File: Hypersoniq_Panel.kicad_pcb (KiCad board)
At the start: 2 copper layers, 40.4 x 128.5 mm, 17 parts

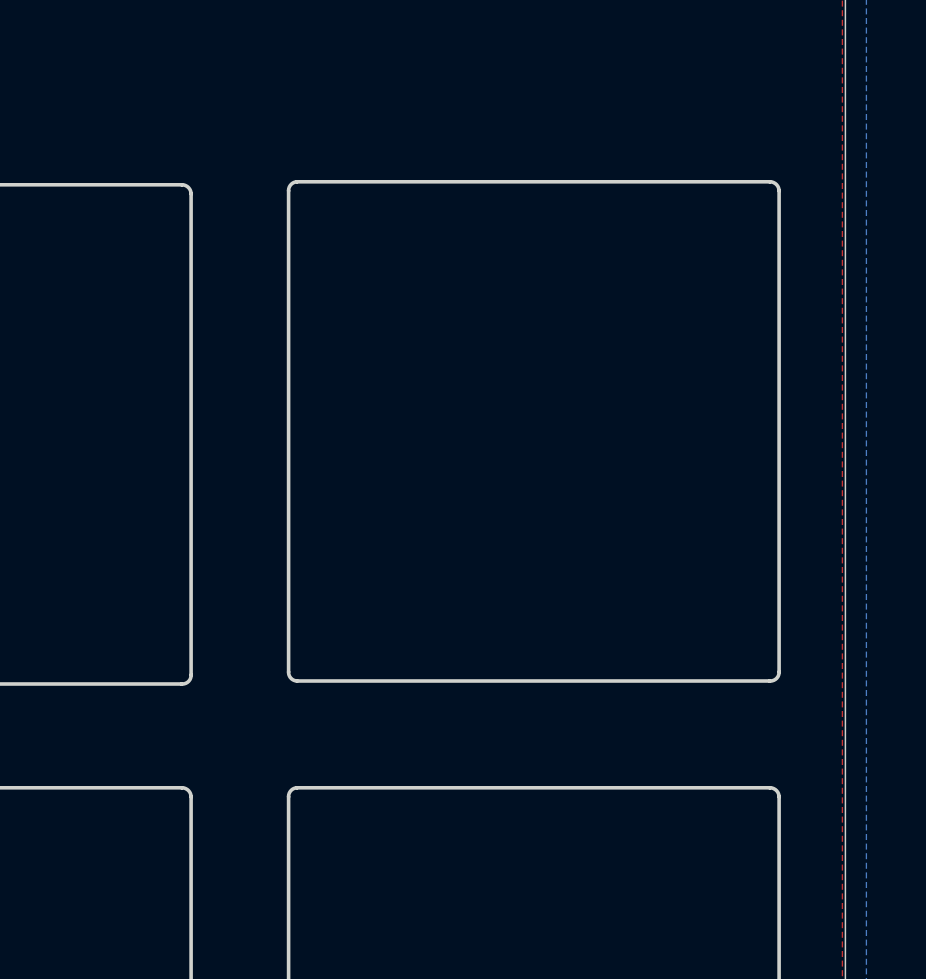
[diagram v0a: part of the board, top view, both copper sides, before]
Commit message: Panel and Control tidy up
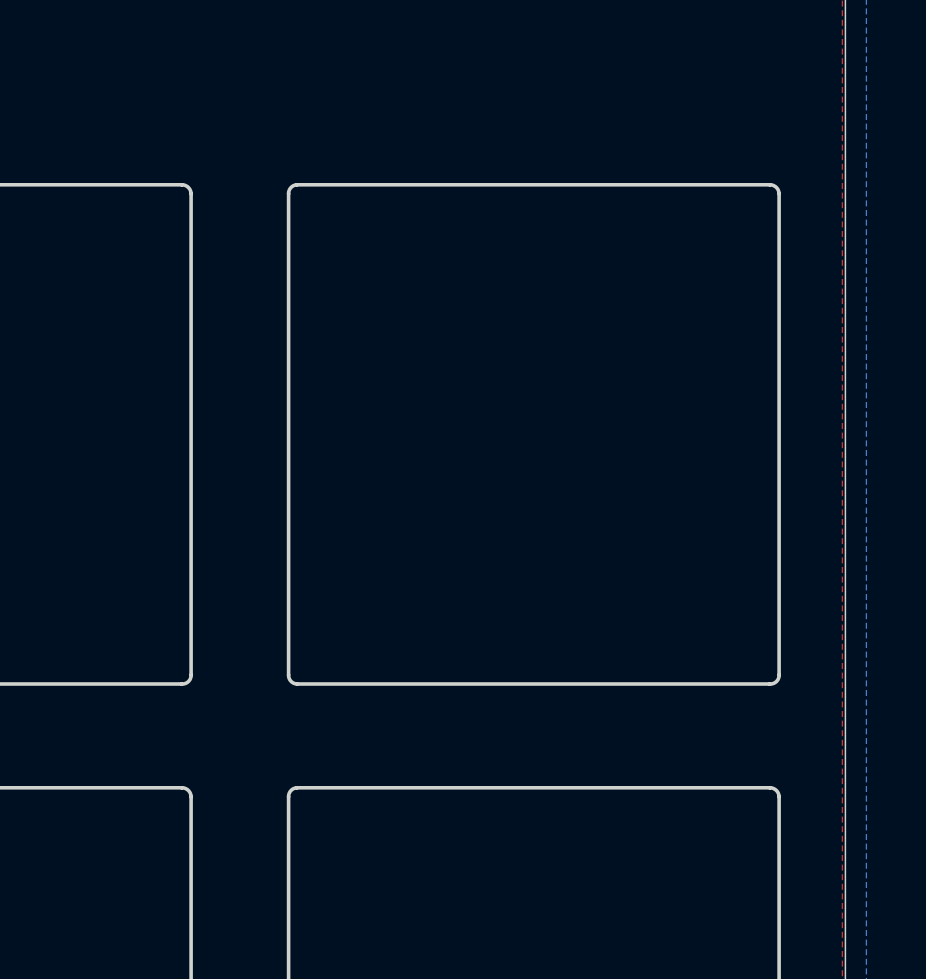
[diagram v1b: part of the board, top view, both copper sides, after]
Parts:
- removed kibuzzard-64BD3DD7: G***, kibuzzard-64BD3DD7
- removed kibuzzard-64BD4829: G***, kibuzzard-64BD4829
- added kibuzzard-64BFAFE6: G***, kibuzzard-64BFAFE6, F.Cu at (79.8, 80.9)
- added kibuzzard-64BFB036: G***, kibuzzard-64BFB036, F.Cu at (70.2, 152.4)
- moved kibuzzard-63FBCCA9 0.50 mm to (56.1, 91.3)
- moved PWM_In 0.10 mm to (80.0, 104.0)

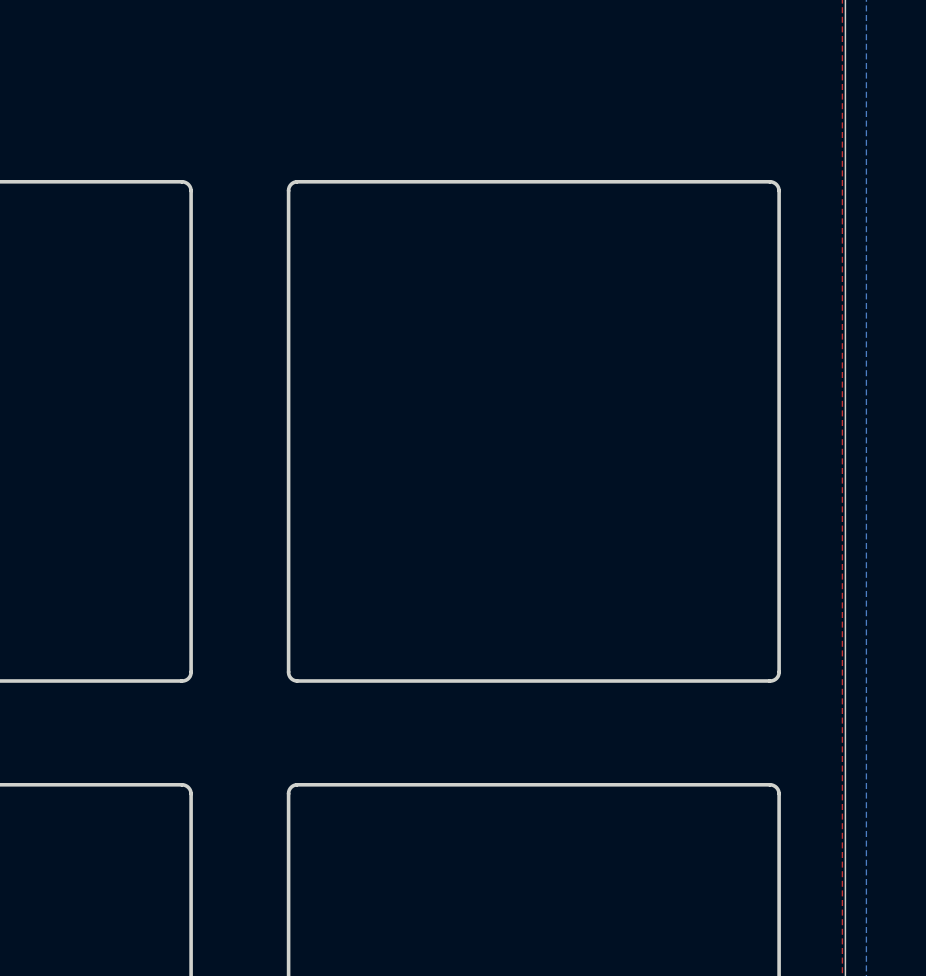
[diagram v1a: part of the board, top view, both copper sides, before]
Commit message: v1.0 Design sent for manufacture
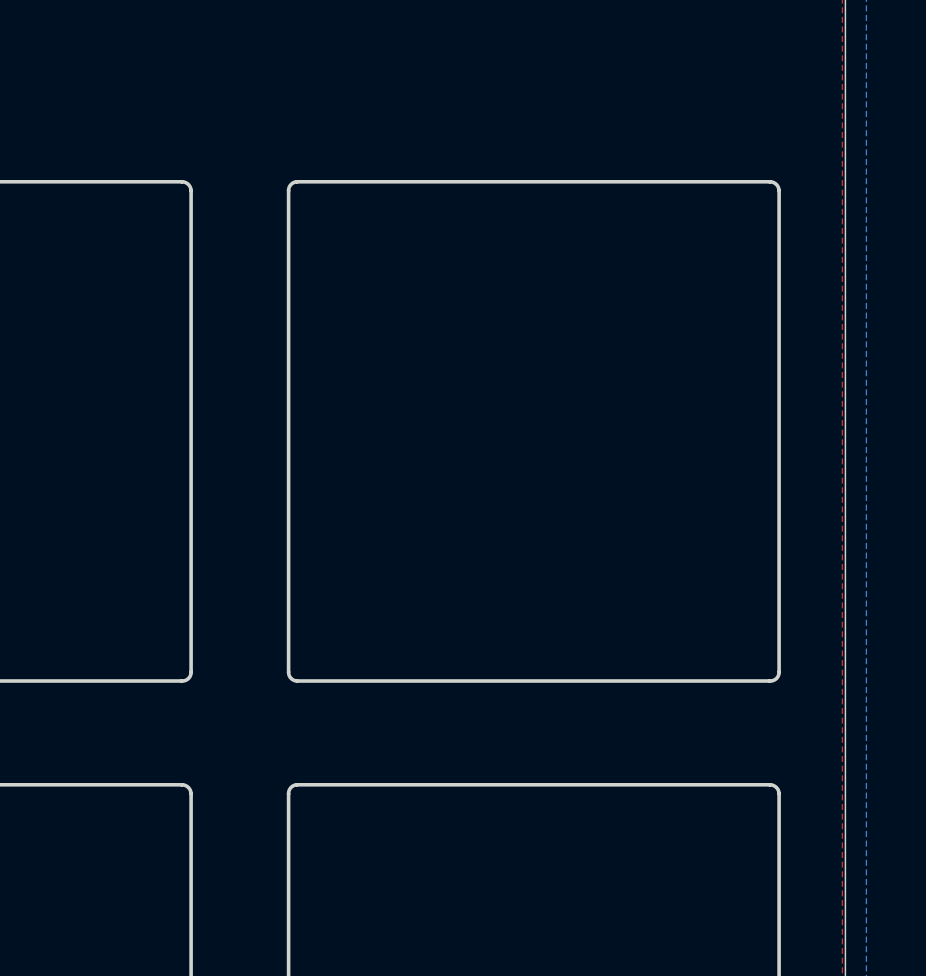
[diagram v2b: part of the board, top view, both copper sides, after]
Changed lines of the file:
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@@
     (pad_to_mask_clearance 0)
     (pcbplotparams
-      (layerselection 0x00010fc_ffffffff)
+      (layerselection 0x00010f0_ffffffff)
       (plot_on_all_layers_selection 0x0000000_00000000)
       (disableapertmacros false)
@@
       (drillshape 0)
       (scaleselection 1)
-      (outputdirectory "Gerbers/Panel/")
+      (outputdirectory "Gerbers/Hypersoniq_Panel/")
     )
   )
@@
     (attr board_only exclude_from_pos_files exclude_from_bom)
     (fp_text reference "kibuzzard-64BFB036" (at 0 -5.432247 90) (layer "F.SilkS") hide
-        (effects (font (size 0 0)))
+        (effects (font (size 0 0) (thickness 0.15)))
     )
     (fp_text value "G***" (at 0 5.432247 90) (layer "F.SilkS") hide
-        (effects (font (size 0 0)))
+        (effects (font (size 0 0) (thickness 0.15)))
     )
     (fp_poly
@@
     (fp_arc (start -7.88 8.32) (mid -8.081749 8.227632) (end -8.16 8.02)
       (stroke (width 0.12) (type solid)) (layer "Edge.Cuts"))
-    (fp_arc (start 7.88 -8.32) (mid 8.096588 -8.233658) (end 8.19 -8.02)
+    (fp_arc (start 7.88 -8.32) (mid 8.096622 -8.233665) (end 8.19 -8.02)
       (stroke (width 0.12) (type solid)) (layer "Edge.Cuts"))
     (fp_arc (start 8.19 8.02) (mid 8.100917 8.238111) (end 7.88 8.32)
@@
     (fp_arc (start -7.88 8.32) (mid -8.081749 8.227632) (end -8.16 8.02)
       (stroke (width 0.12) (type solid)) (layer "Edge.Cuts"))
-    (fp_arc (start 7.88 -8.32) (mid 8.096588 -8.233658) (end 8.19 -8.02)
+    (fp_arc (start 7.88 -8.32) (mid 8.096622 -8.233665) (end 8.19 -8.02)
       (stroke (width 0.12) (type solid)) (layer "Edge.Cuts"))
     (fp_arc (start 8.19 8.02) (mid 8.100917 8.238111) (end 7.88 8.32)
@@
     (fp_arc (start -7.88 8.32) (mid -8.081749 8.227632) (end -8.16 8.02)
       (stroke (width 0.12) (type solid)) (layer "Edge.Cuts"))
-    (fp_arc (start 7.88 -8.32) (mid 8.096588 -8.233658) (end 8.19 -8.02)
+    (fp_arc (start 7.88 -8.32) (mid 8.096622 -8.233665) (end 8.19 -8.02)
       (stroke (width 0.12) (type solid)) (layer "Edge.Cuts"))
     (fp_arc (start 8.19 8.02) (mid 8.100917 8.238111) (end 7.88 8.32)
@@
     (fp_arc (start -7.88 8.32) (mid -8.081749 8.227632) (end -8.16 8.02)
       (stroke (width 0.12) (type solid)) (layer "Edge.Cuts"))
-    (fp_arc (start 7.88 -8.32) (mid 8.096588 -8.233658) (end 8.19 -8.02)
+    (fp_arc (start 7.88 -8.32) (mid 8.096622 -8.233665) (end 8.19 -8.02)
       (stroke (width 0.12) (type solid)) (layer "Edge.Cuts"))
     (fp_arc (start 8.19 8.02) (mid 8.100917 8.238111) (end 7.88 8.32)
@@
     (attr board_only exclude_from_pos_files exclude_from_bom)
     (fp_text reference "kibuzzard-64BFAFE6" (at 0 -5.294375 90) (layer "F.SilkS") hide
-        (effects (font (size 0 0)))
+        (effects (font (size 0 0) (thickness 0.15)))
     )
     (fp_text value "G***" (at 0 5.294375 90) (layer "F.SilkS") hide
-        (effects (font (size 0 0)))
-    )
-    (fp_poly
+        (effects (font (size 0 0) (thickness 0.15)))
+    )
+    (fp_poly
